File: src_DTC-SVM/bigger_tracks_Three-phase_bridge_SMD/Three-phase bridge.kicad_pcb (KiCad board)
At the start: 2 copper layers, 401.6 x 318 mm, 105 parts, among them M1 MCP6022-I/P, M2 MCP6022-I/P, P1 CONN_1, P10 CONN_1, P11 CONN_1, P12 CONN_1, P13 CONN_1, P2 POWER_FUSE, P3 CONN_2, P4 CONN_1, P5 CONN_1, P6 POWER_FUSE, P7 CONN_1, P8 CONN_1, P9 CONN_1

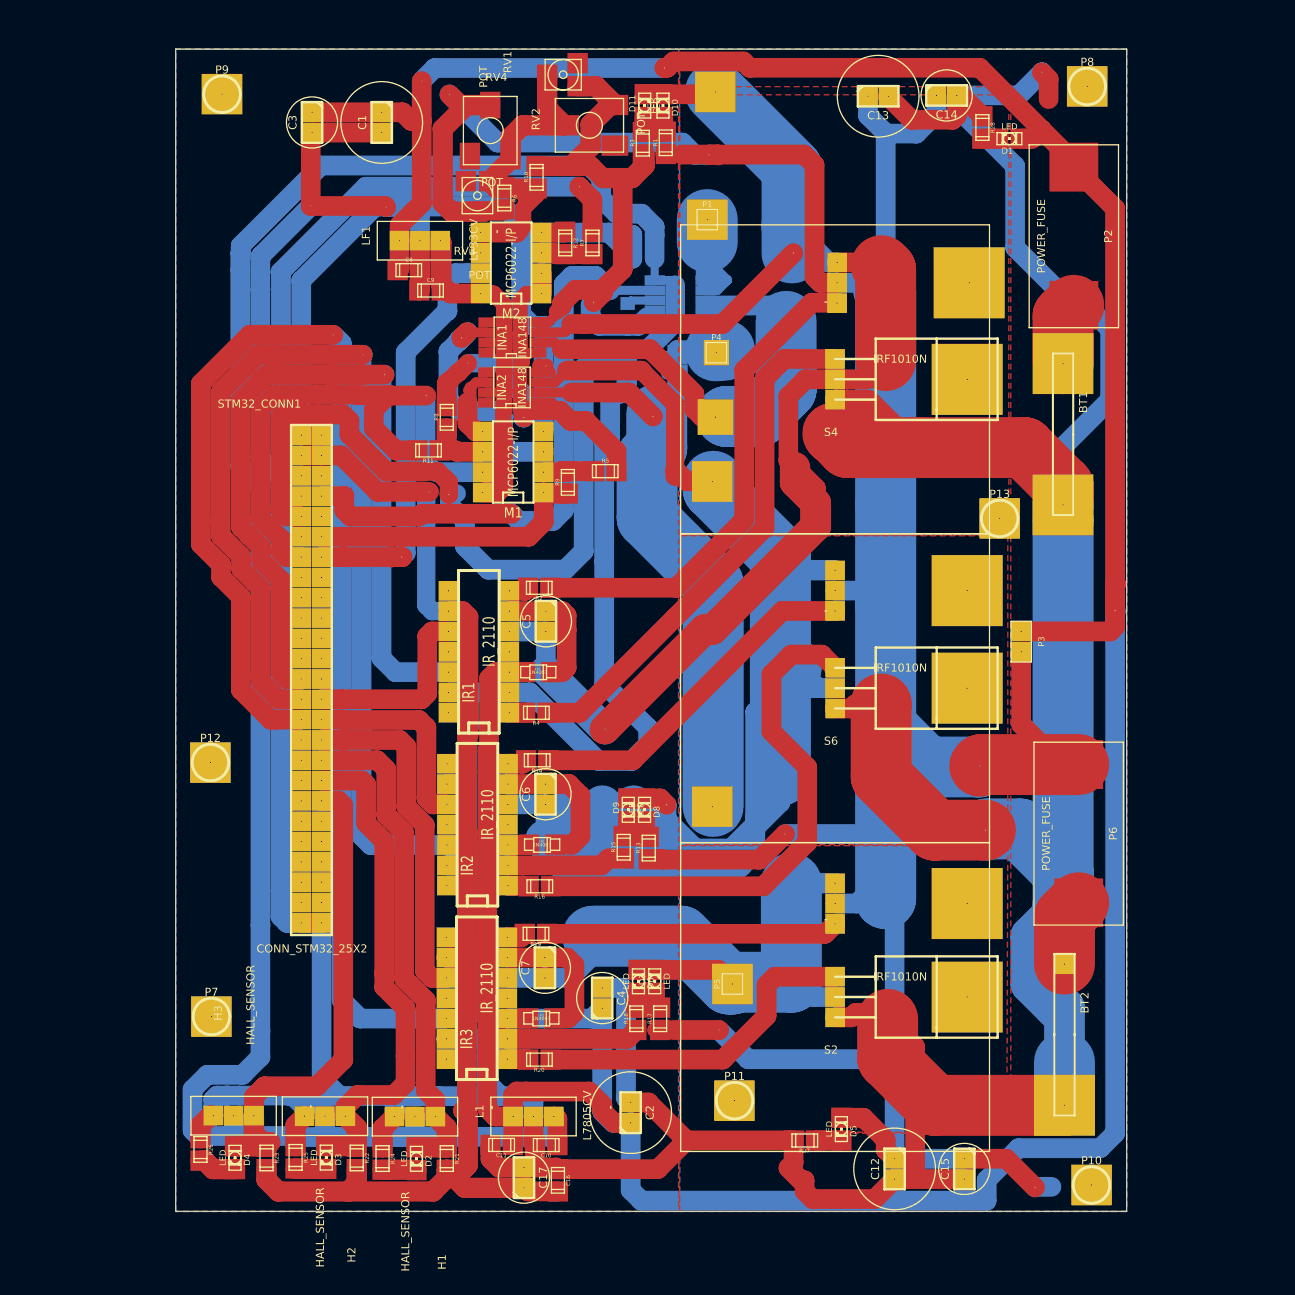
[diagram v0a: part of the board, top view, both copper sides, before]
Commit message: PCB base movil parte Sebastian LISTA
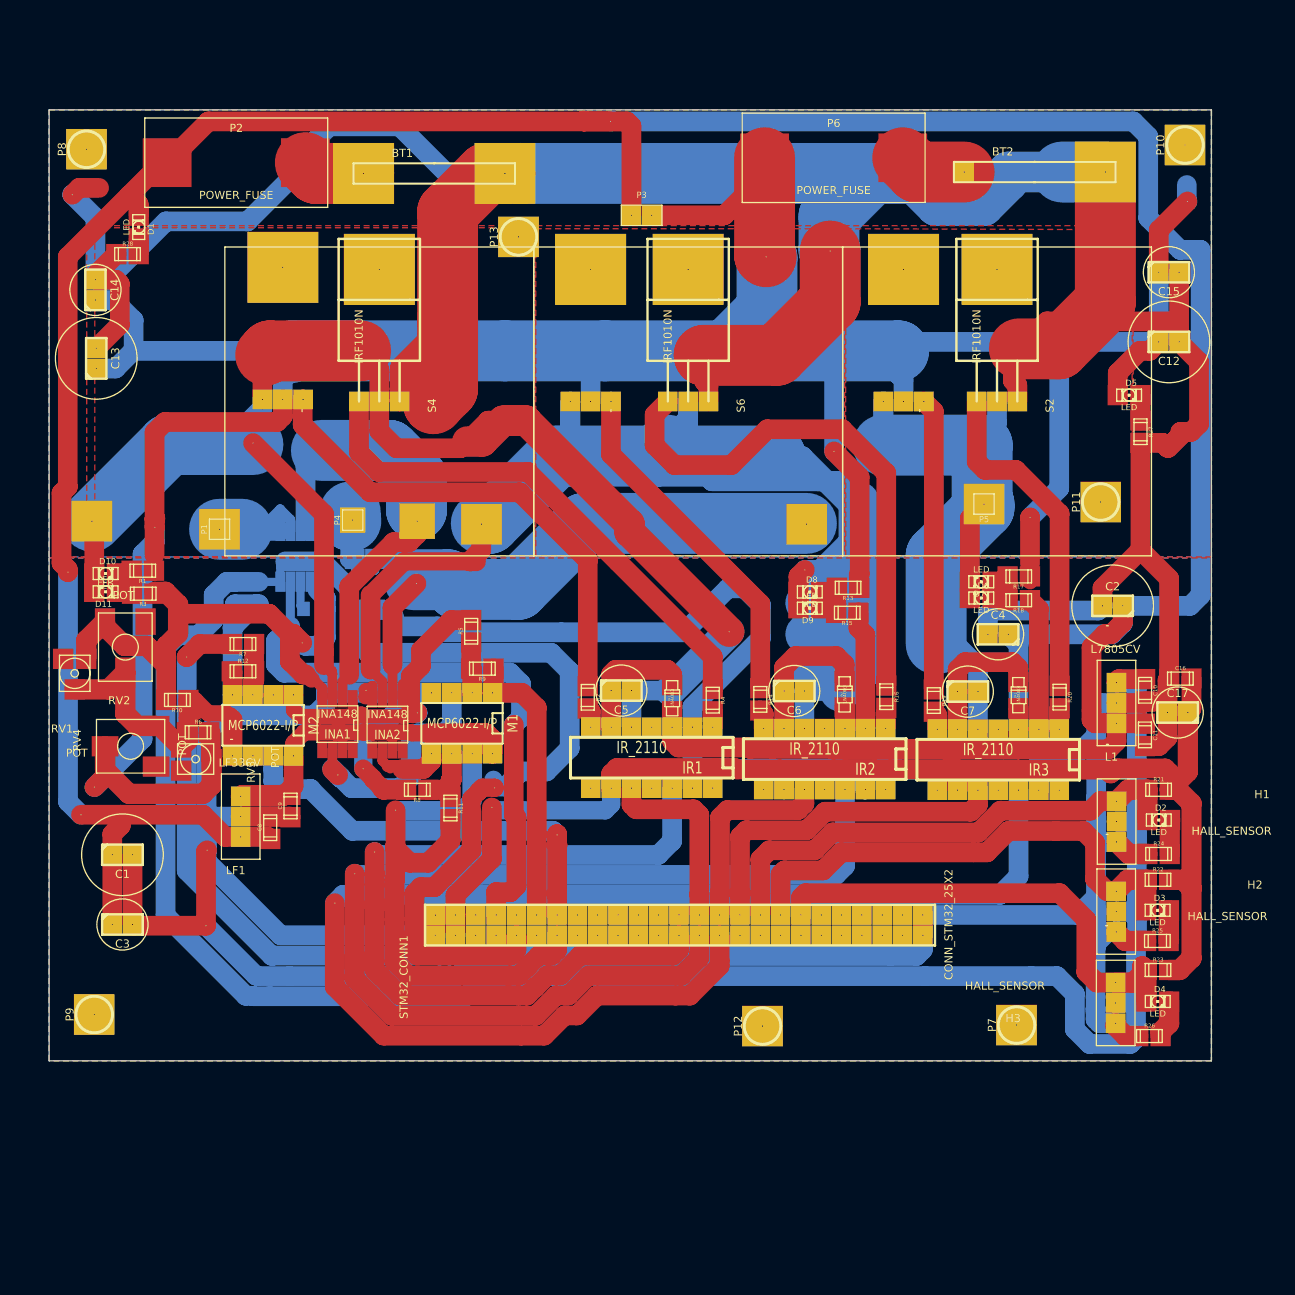
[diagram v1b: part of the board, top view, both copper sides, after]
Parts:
- moved P10 130.5 mm to (283.1, 76.5), turned to 90 degrees
- moved P8 125.3 mm to (145.8, 77.0), turned to 90 degrees
- moved R26 119.5 mm to (278.7, 187.9), turned to 0 degrees
- moved D4 117.0 mm to (279.7, 183.6), turned to 0 degrees
- moved P9 116.1 mm to (146.8, 185.2), turned to 90 degrees
- moved C15 115.0 mm to (281.1, 92.4), turned to 0 degrees
- moved R23 113.9 mm to (279.8, 179.6), turned to 0 degrees
- moved H3 111.2 mm to (274.5, 183.7), turned to 0 degrees
- moved R25 111.1 mm to (279.7, 176.0), turned to 0 degrees
- moved D1 109.4 mm to (152.3, 86.8), turned to 270 degrees
- moved C14 109.1 mm to (146.9, 94.6), turned to 90 degrees
- moved C12 108.9 mm to (281.1, 101.1), turned to 0 degrees
- moved BT2 108.6 mm to (265.0, 79.9), turned to 0 degrees
- moved D3 108.4 mm to (279.7, 172.2), turned to 0 degrees
- moved R28 108.0 mm to (151.0, 90.1), turned to 0 degrees
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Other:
- board size 401.6 x 318 mm -> 412.2 x 299.2 mm
